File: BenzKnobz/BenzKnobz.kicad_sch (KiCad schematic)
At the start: 40 parts, among them J1 Barrel_Jack, J10 I2C_STANDARDJS-1MM, J11 Conn_01x02, J12 Conn_01x07, J13 Conn_01x07, J14 Conn_01x07, J15 Conn_01x07, J16 Conn_01x07, J17 Conn_01x07, J18 Conn_01x07, J2 MIDI OUT, J3 MIDI IN, J4 MJ-3502, J5 MJ-3502, J6 MJ-3502, J7 MJ-3502, J8 MJ-3502, J9 MJ-3502, SW7 SW_Push_SPDT, U1 teensy 4.0, U10 6N138, U11 LM317_TO-220, U12 CD74HC4050E, U2 CD74HC4050E, U3 74HC4051, U4 74HC4051, U5 74HC4051, U6 74HC4051, U7 74HC4051, U8 74HC4051, U9 74HC4051

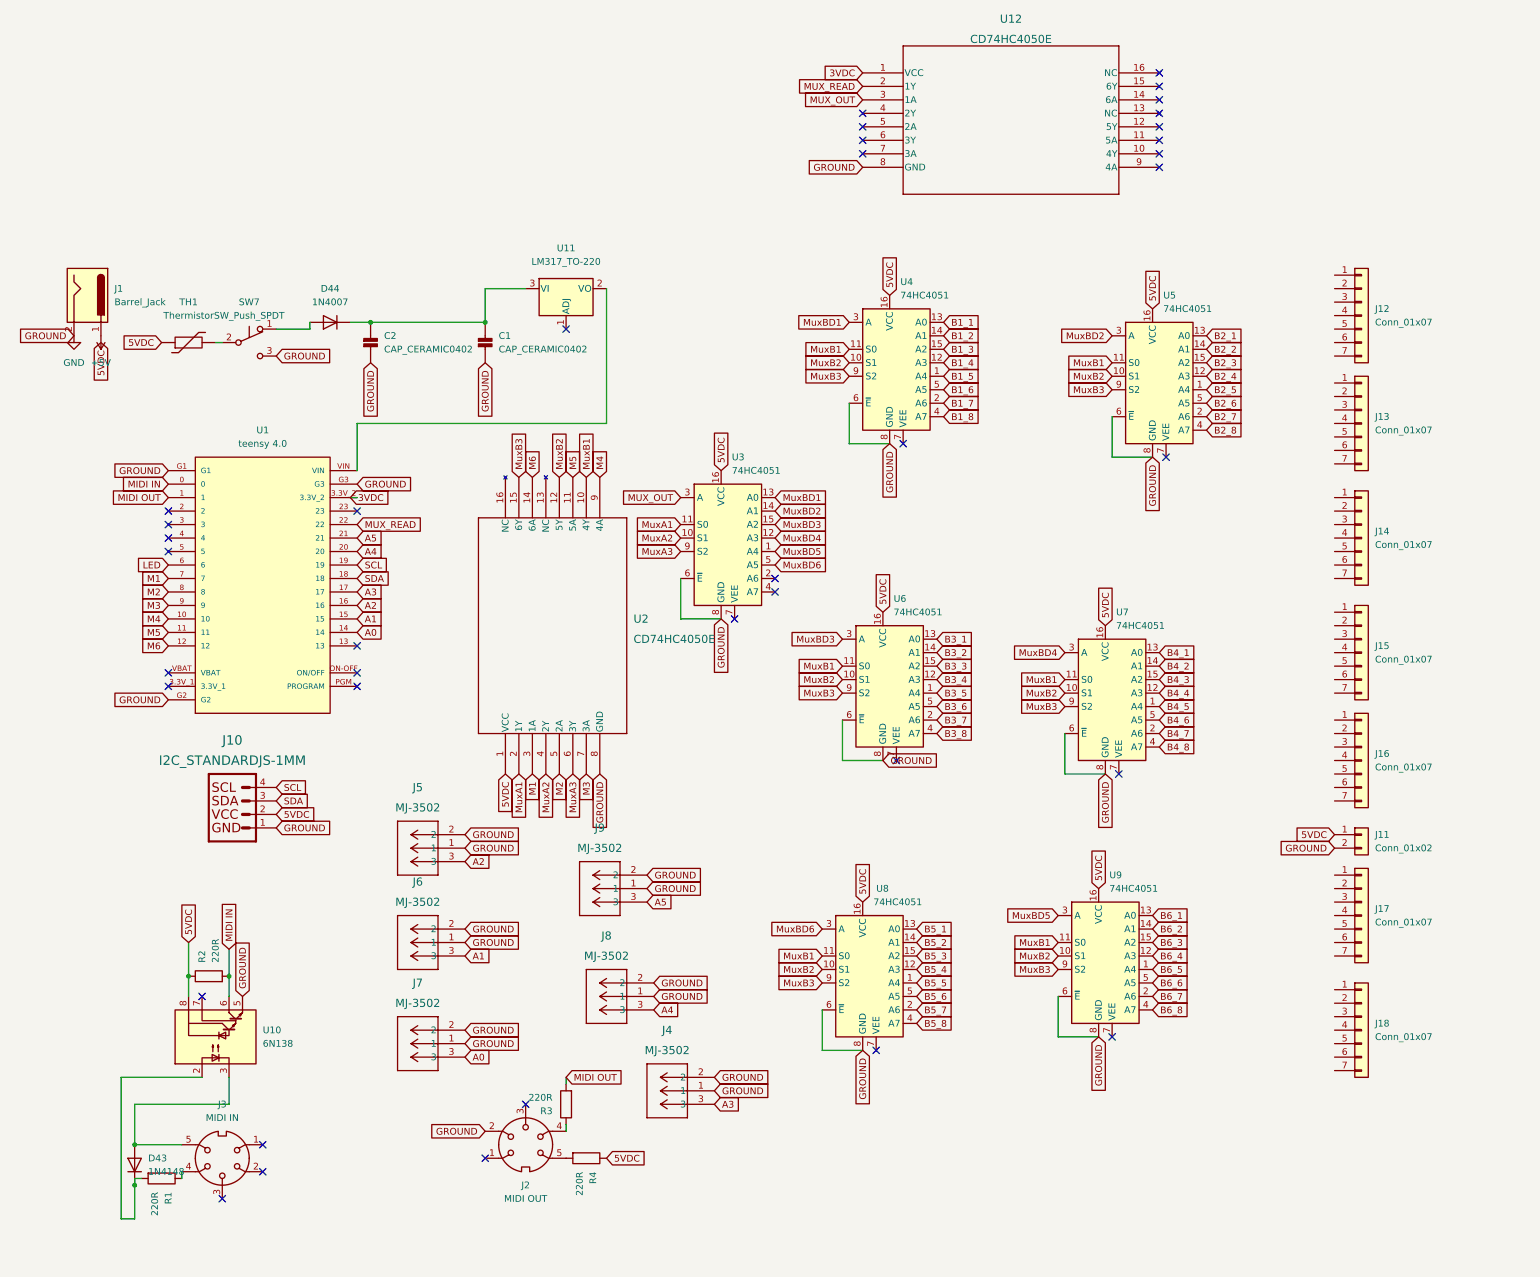
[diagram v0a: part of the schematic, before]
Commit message: brd
moar - almost completely laid out
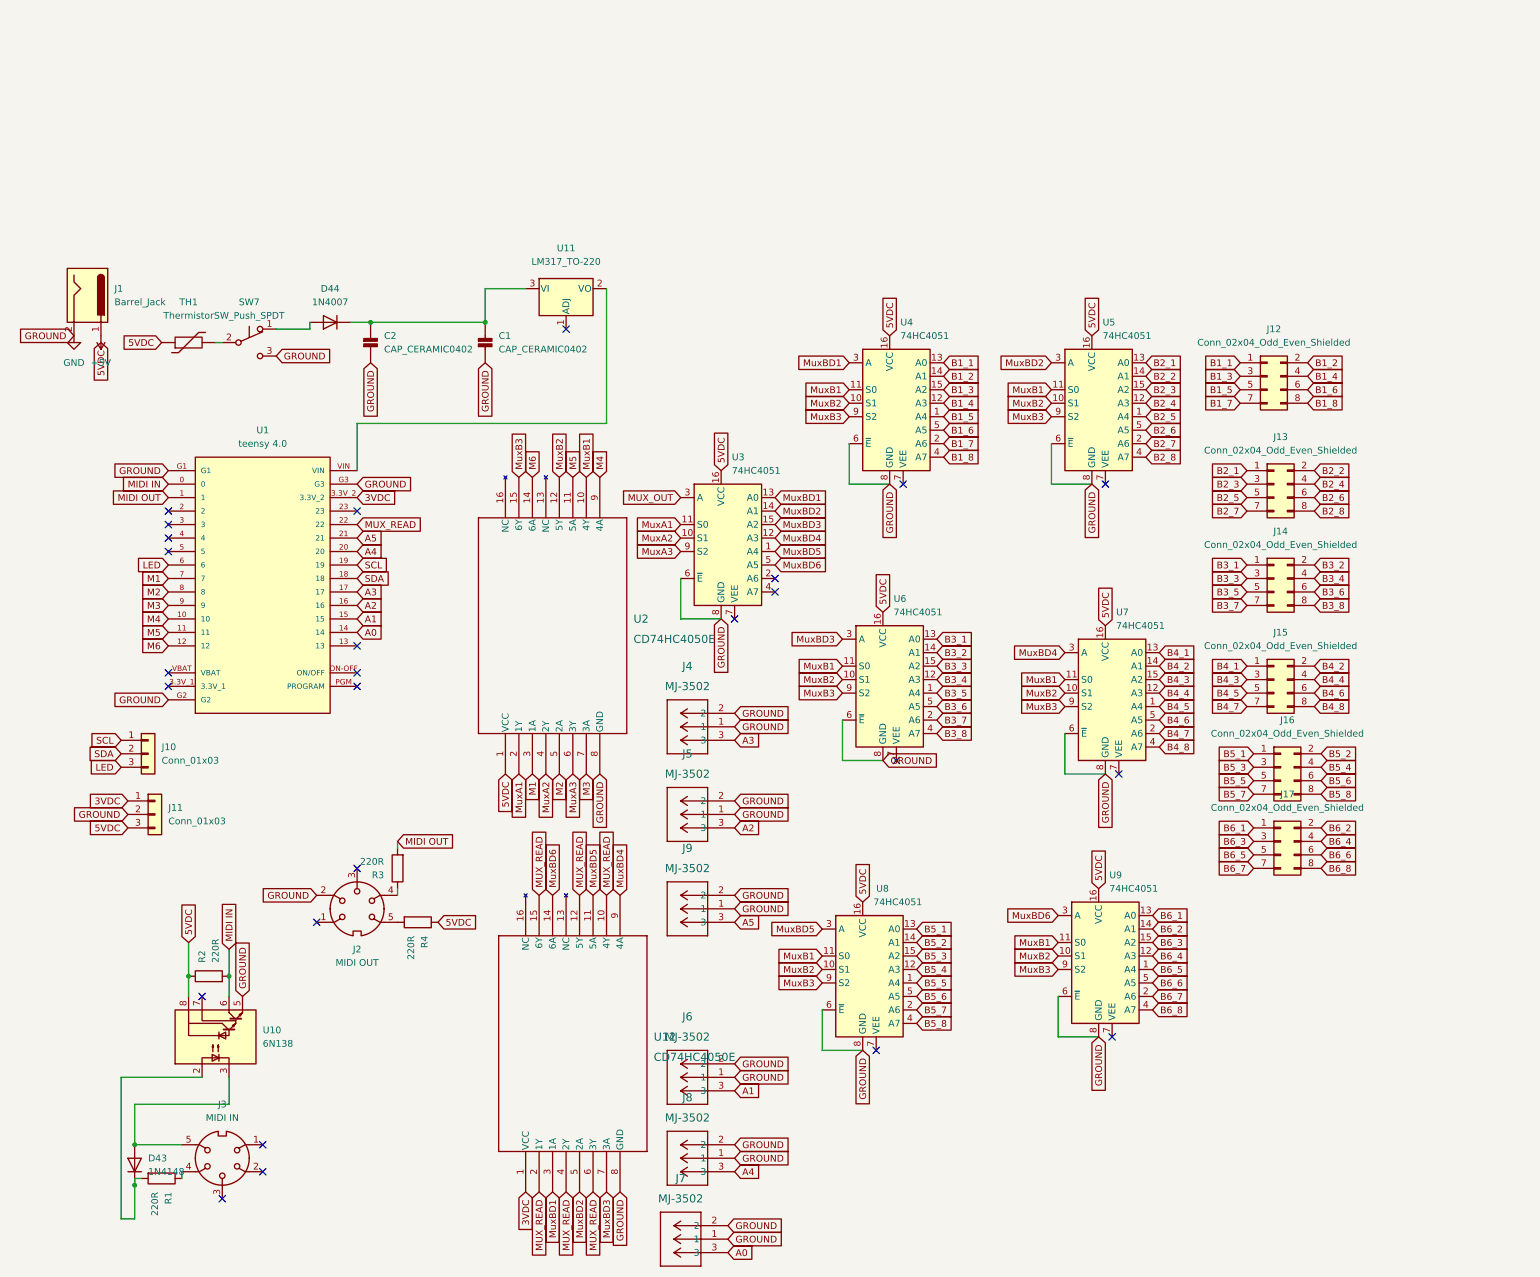
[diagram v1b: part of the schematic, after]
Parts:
- removed J10: I2C_STANDARDJS-1MM, Connector_JST:JST_EH_S4B-EH_1x04_P2.50mm_Horizontal, symbol Qwiic_OLED_1.3in-eagle-import:I2C_STANDARDJS-1MM
- removed J11: Conn_01x02, Connector_PinHeader_1.00mm:PinHeader_1x02_P1.00mm_Vertical, symbol Connector_Generic:Conn_01x02
- removed J12, J13, J14, J15, J16, J17, J18: Conn_01x07, Connector_PinHeader_1.00mm:PinHeader_1x07_P1.00mm_Vertical, symbol Connector_Generic:Conn_01x07
- added J10, J11: Conn_01x03, Connector_PinHeader_1.00mm:PinHeader_1x03_P1.00mm_Vertical, symbol Connector_Generic:Conn_01x03
- added J12, J13, J14, J15, J16, J17: Conn_02x04_Odd_Even_Shielded, Connector_PinHeader_1.00mm:PinHeader_2x04_P1.00mm_Vertical, symbol Connector_Generic:Conn_02x04_Odd_Even
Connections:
- net 3VDC: now also J11.1 (Pin_1)
- net 5VDC: now also J11.3 (Pin_3)
- net B1_1: now also J12.1 (Pin_1)
- net B1_2: now also J12.2 (Pin_2)
- net B1_3: now also J12.3 (Pin_3)
- net B1_4: now also J12.4 (Pin_4)
- net B1_5: now also J12.5 (Pin_5)
- net B1_6: now also J12.6 (Pin_6)
- net B1_7: now also J12.7 (Pin_7)
- net B1_8: now also J12.8 (Pin_8)
- net B2_1: now also J13.1 (Pin_1)
- net B2_2: now also J13.2 (Pin_2)
- net B2_3: now also J13.3 (Pin_3)
- net B2_4: now also J13.4 (Pin_4)
- net B2_5: now also J13.5 (Pin_5)
- net B2_6: now also J13.6 (Pin_6)
- net B2_7: now also J13.7 (Pin_7)
- net B2_8: now also J13.8 (Pin_8)
- net B3_1: now also J14.1 (Pin_1)
- net B3_2: now also J14.2 (Pin_2)
- net B3_3: now also J14.3 (Pin_3)
- net B3_4: now also J14.4 (Pin_4)
- net B3_5: now also J14.5 (Pin_5)
- net B3_6: now also J14.6 (Pin_6)
- net B3_7: now also J14.7 (Pin_7)
- net B3_8: now also J14.8 (Pin_8)
- net B4_1: now also J15.1 (Pin_1)
- net B4_2: now also J15.2 (Pin_2)
- net B4_3: now also J15.3 (Pin_3)
- net B4_4: now also J15.4 (Pin_4)
- net B4_5: now also J15.5 (Pin_5)
- net B4_6: now also J15.6 (Pin_6)
- net B4_7: now also J15.7 (Pin_7)
- net B4_8: now also J15.8 (Pin_8)
- net B5_1: now also J16.1 (Pin_1)
- net B5_2: now also J16.2 (Pin_2)
- net B5_3: now also J16.3 (Pin_3)
- net B5_4: now also J16.4 (Pin_4)
- net B5_5: now also J16.5 (Pin_5)
- net B5_6: now also J16.6 (Pin_6)
- net B5_7: now also J16.7 (Pin_7)
- net B5_8: now also J16.8 (Pin_8)
- net B6_1: now also J17.1 (Pin_1)
- net B6_2: now also J17.2 (Pin_2)
- net B6_3: now also J17.3 (Pin_3)
- net B6_4: now also J17.4 (Pin_4)
- net B6_5: now also J17.5 (Pin_5)
- net B6_6: now also J17.6 (Pin_6)
- net B6_7: now also J17.7 (Pin_7)
- net B6_8: now also J17.8 (Pin_8)
- net GND: now also J11.2 (Pin_2)
- net LED: now also J10.3 (Pin_3)
- net MUX_OUT: no longer U12.3 (1A)
- net MUX_READ: now also U12.10 (4Y), U12.12 (5Y), U12.15 (6Y), U12.4 (2Y), U12.6 (3Y)
- net MuxBD1: now also U12.3 (1A)
- net MuxBD2: now also U12.5 (2A)
- net MuxBD3: now also U12.7 (3A)
- net MuxBD4: now also U12.9 (4A)
- net MuxBD5: now also U12.11 (5A), U8.3 (A); no longer U9.3 (A)
- net MuxBD6: now also U12.14 (6A), U9.3 (A); no longer U8.3 (A)
- net SCL: now also J10.1 (Pin_1)
- net SDA: now also J10.2 (Pin_2)
- no-connect marks 39 -> 27
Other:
- moved on the sheet: J2, J4, J5, J6, J7, J8, J9, R3, R4, U4, U5
